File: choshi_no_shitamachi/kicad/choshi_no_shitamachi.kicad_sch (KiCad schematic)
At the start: 5 parts, among them J1 Analog, J2 Digital

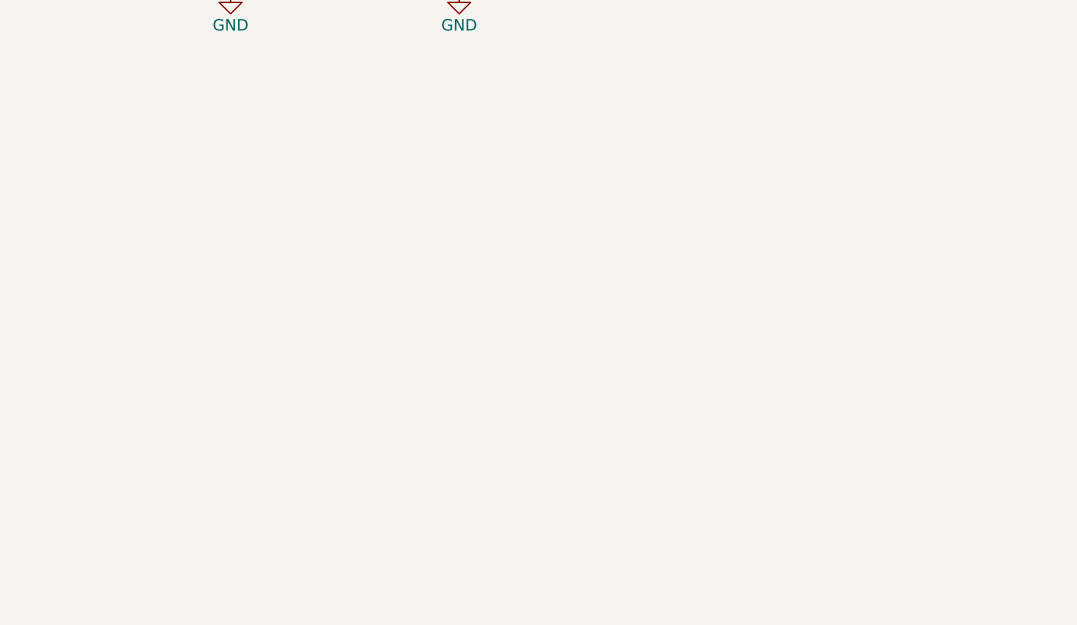
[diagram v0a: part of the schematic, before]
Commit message: vibe-coded schematic test
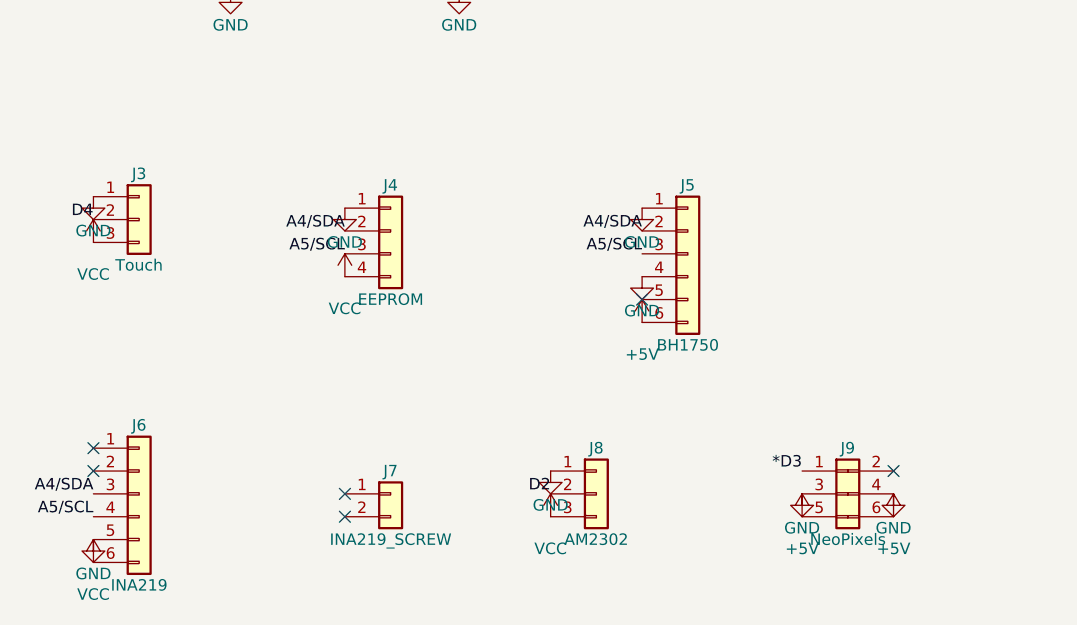
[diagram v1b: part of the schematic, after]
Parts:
- added J3: Touch, Connector_PinHeader_2.54mm:PinHeader_1x03_P2.54mm_Vertical, symbol Connector_Generic:Conn_01x03
- added J4: EEPROM, Connector_PinHeader_2.54mm:PinHeader_1x04_P2.54mm_Vertical, symbol Connector_Generic:Conn_01x04
- added J5: BH1750, Connector_PinHeader_2.54mm:PinHeader_1x06_P2.54mm_Vertical, symbol Connector_Generic:Conn_01x06
- added J6: INA219, Connector_PinHeader_2.54mm:PinHeader_1x06_P2.54mm_Vertical, symbol Connector_Generic:Conn_01x06
- added J7: INA219_SCREW, Connector_PinHeader_2.54mm:PinHeader_1x02_P2.54mm_Vertical, symbol Connector_Generic:Conn_01x02
- added J8: AM2302, Connector_PinHeader_2.54mm:PinHeader_1x03_P2.54mm_Vertical, symbol Connector_Generic:Conn_01x03
- added J9: NeoPixels, Connector_PinHeader_2.54mm:PinHeader_2x03_P2.54mm_Vertical_OddEven, symbol Connector_Generic:Conn_02x03_Odd_Even
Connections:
- net *D3: now also J9.1 (Pin_1)
- net +5V: now also J5.6 (Pin_6), J9.5 (Pin_5), J9.6 (Pin_6)
- net A4/SDA: now also J4.2 (Pin_2), J5.2 (Pin_2), J6.3 (Pin_3)
- net A5/SCL: now also J4.3 (Pin_3), J5.3 (Pin_3), J6.4 (Pin_4)
- net D2: now also J8.2 (Pin_2)
- net D4: now also J3.2 (Pin_2)
- net GND: now also J3.1 (Pin_1), J4.1 (Pin_1), J5.1 (Pin_1), J5.4 (Pin_4), J6.5 (Pin_5), J8.1 (Pin_1), J9.3 (Pin_3), J9.4 (Pin_4)
- net VCC: now also J3.3 (Pin_3), J4.4 (Pin_4), J6.6 (Pin_6), J8.3 (Pin_3)
- no-connect marks 0 -> 6
